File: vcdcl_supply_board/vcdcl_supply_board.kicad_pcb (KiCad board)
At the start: 2 copper layers, 30 x 50 mm, 19 parts, among them J1 Conn_01x02_Male, Q1 IRFR9024, Q2 Q_NPN_ECB, Q3 Q_NPN_BCE, SW1 SW_DIP_x01

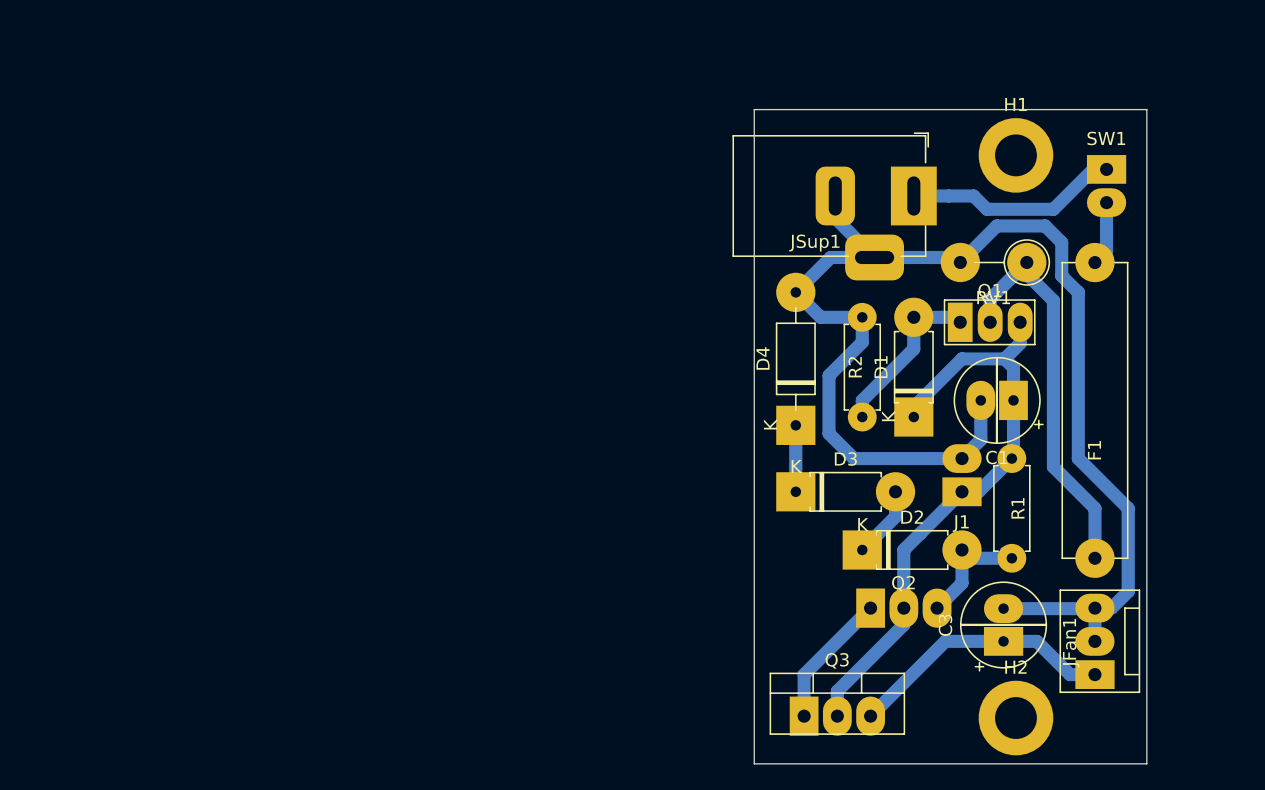
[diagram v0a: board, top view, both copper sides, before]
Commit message: Supply board fixes
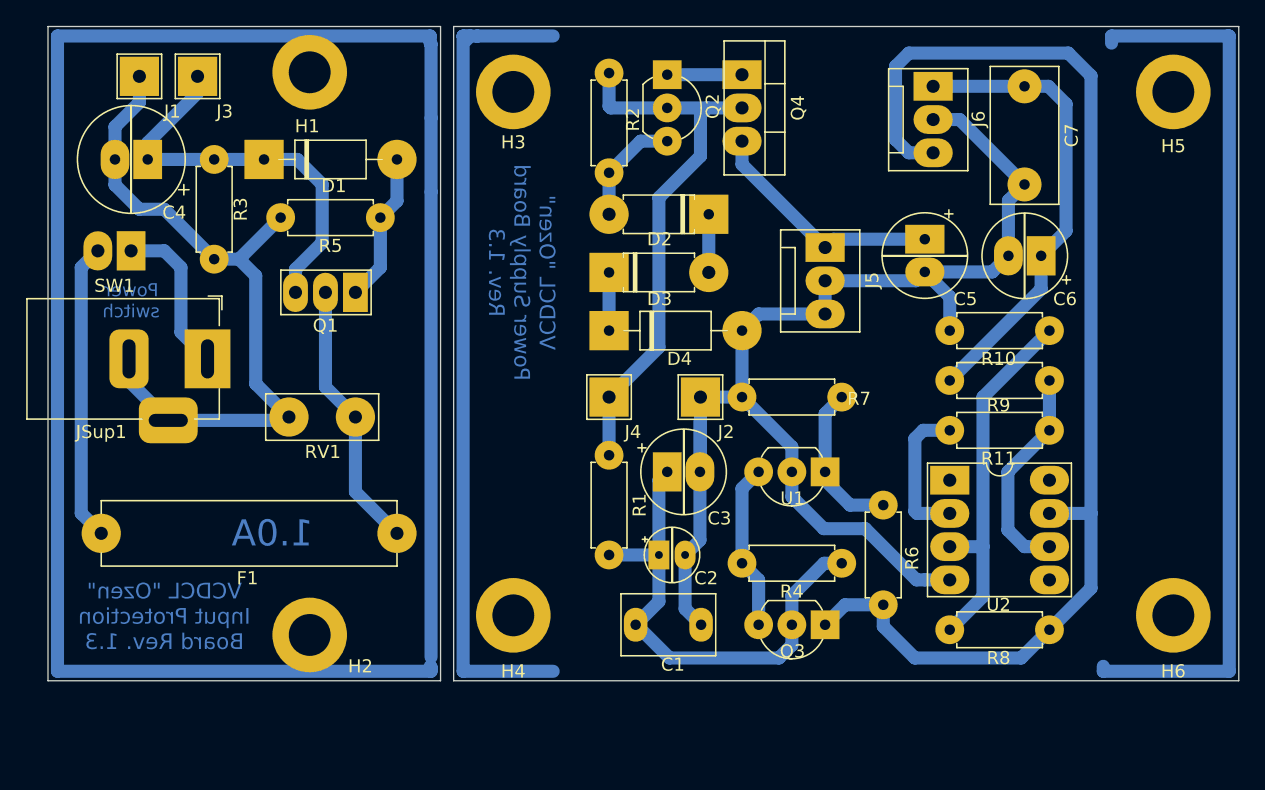
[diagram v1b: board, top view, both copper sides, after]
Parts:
- removed JFan1: Conn_01x03, _сustom:LUT_FanPinHeader_1x03_P2.54mm_Vertical
- added C2: 10u, _сustom:LUT_CP_Radial_D4.0mm_P2.00mm, F.Cu at (72.7, 64.0)
- added C4: 47u 63v, _сustom:LUT_CP_Radial_D8.0mm_P2.50mm, F.Cu at (33.6, 33.8)
- added C5: 470u 16v, _сustom:LUT_CP_Radial_D6.3mm_P2.50mm, F.Cu at (93.0, 39.9)
- added C6: 470u, _сustom:LUT_CP_Radial_D6.3mm_P2.50mm, F.Cu at (101.9, 41.2)
- added C7: 150u, _сustom:LUT_C_Rect_L10.3mm_W5.0mm_P7.50mm, F.Cu at (100.7, 28.2)
- added G***: LOGO, _сustom:Logo_Ozen_7.0x9.0, F.Cu at (62.9, 59.8)
- added G***: LOGO, _сustom:Logo_Ozen_7.0x9.0, F.Cu at (34.9, 60.5)
- added H3: MountingHole_Pad, MountingHole:MountingHole_3.2mm_M3_ISO7380_Pad, F.Cu at (61.6, 28.6)
- added H4: MountingHole_Pad, MountingHole:MountingHole_3.2mm_M3_ISO7380_Pad, F.Cu at (61.6, 68.7)
- added H5: MountingHole_Pad, MountingHole:MountingHole_3.2mm_M3_ISO7380_Pad, F.Cu at (112.0, 28.6)
- added H6: MountingHole_Pad, MountingHole:MountingHole_3.2mm_M3_ISO7380_Pad, F.Cu at (112.0, 68.7)
- added J2: Conn_01x01_Female, _сustom:LUT_PinHeader_1x01_P2.54mm_Vertical, F.Cu at (75.9, 52.0)
- added J3: Conn_01x01_Female, _сustom:LUT_PinHeader_1x01_P2.54mm_Vertical, F.Cu at (37.5, 27.5)
- added J4: Conn_01x01_Female, _сustom:LUT_PinHeader_1x01_P2.54mm_Vertical, F.Cu at (68.9, 52.0)
- added J5: Conn_01x03, _сustom:LUT_FanPinHeader_1x03_P2.54mm_Vertical, F.Cu at (85.4, 40.5)
- added J6: Conn_01x03, _сustom:LUT_FanPinHeader_1x03_P2.54mm_Vertical, F.Cu at (93.7, 28.2)
- added Q4: Q_NPN_BCE, _сustom:LUT_TO-220-3_Vertical, F.Cu at (79.1, 27.3)
- added R10: 5k 1%, _сustom:LUT_R_L6.3mm_D2.5mm_P7.62mm_Horizontal, F.Cu at (102.6, 46.9)
- added R11: 5k, _сustom:LUT_R_L6.3mm_D2.5mm_P7.62mm_Horizontal, F.Cu at (102.6, 54.5)
- added R3: 100k, _сustom:LUT_R_L6.3mm_D2.5mm_P7.62mm_Horizontal, F.Cu at (38.7, 41.4)
- added R4: 1k, _сustom:LUT_R_L6.3mm_D2.5mm_P7.62mm_Horizontal, F.Cu at (86.7, 64.7)
- added R5: 5k, _сustom:LUT_R_L6.3mm_D2.5mm_P7.62mm_Horizontal, F.Cu at (51.4, 38.3)
- added R6: 5k 1%, _сustom:LUT_R_L6.3mm_D2.5mm_P7.62mm_Horizontal, F.Cu at (89.9, 67.8)
- added R7: 1k 1%, _сustom:LUT_R_L6.3mm_D2.5mm_P7.62mm_Horizontal, F.Cu at (86.7, 52.0)
- added R8: 10k 1%, _сustom:LUT_R_L6.3mm_D2.5mm_P7.62mm_Horizontal, F.Cu at (102.6, 69.8)
- added R9: 47, _сustom:LUT_R_L6.3mm_D2.5mm_P7.62mm_Horizontal, F.Cu at (94.9, 50.7)
- added U1: TL431LP, _сustom:LUT_TO-92, F.Cu at (85.4, 57.7)
- added U2: LM741, _сustom:LUT_DIP-8, F.Cu at (94.9, 58.3)
- C1: value 100u -> 1u; footprint _сustom:LUT_CP_Radial_D6.3mm_P2.50mm -> _сustom:LUT_C_Rect_L7.0mm_W4.5mm_P5.00mm
- C3: value 470u -> 100u
- D1: footprint _сustom:LUT_D_P7.62mm_Horizontal -> _сustom:LUT_D_P10.16mm_Horizontal
- J1: value Conn_01x02_Male -> Conn_01x01_Female; footprint _сustom:LUT_PinHeader_1x02_P2.54mm_Vertical -> _сustom:LUT_PinHeader_1x01_P2.54mm_Vertical
- Q3: value Q_NPN_BCE -> Q_NPN_ECB; footprint _сustom:LUT_TO-220-3_Vertical -> _сustom:LUT_TO-92
- R1: value 1k -> R
- R2: value 10k -> 390
- moved SW1 74.8 mm to (32.4, 40.8), turned to 270 degrees
- moved J1 70.4 mm to (33.0, 27.5)
- moved JSup1 55.4 mm to (38.2, 49.0)
- moved H1 54.3 mm to (46.0, 27.1)
- moved H2 54.3 mm to (46.0, 70.2)
- moved D1 53.4 mm to (42.5, 33.8), turned to 0 degrees
- moved F1 53.4 mm to (52.7, 62.4), turned to 180 degrees
- moved RV1 52.6 mm to (49.5, 53.5)
- moved Q1 46.3 mm to (49.5, 44.0), turned to 180 degrees
- moved Q2 43.6 mm to (73.3, 27.3), turned to 270 degrees
- moved C1 33.6 mm to (70.9, 69.4), turned to 0 degrees
- moved R2 32.6 mm to (68.9, 27.2), turned to 270 degrees
- moved R1 31.7 mm to (68.9, 64.0), turned to 90 degrees
- moved C3 28.8 mm to (73.3, 57.7), turned to 0 degrees
- moved D2 28.2 mm to (76.5, 38.0), turned to 180 degrees
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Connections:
- C1 pad 1: V+ -> Net-(C1-Pad1)
- C3 pad 1: +12V -> Net-(C1-Pad1)
- D1 pad 1: V+ -> Vin
- J1 pad 1: V+ -> Earth
- Q1 pad 3: V+ -> Vin
- Q2 pad 2: V+ -> Vin
- Q3 pad 1: Net-(Q2-Pad1) -> +15V
- Q3 pad 2: V+ -> Net-(C1-Pad1)
- Q3 pad 3: +12V -> Net-(Q3-Pad3)
- R1 pad 1: V+ -> Net-(C1-Pad1)
- R1 pad 2: Net-(D2-Pad2) -> Vin
- R2 pad 1: Net-(D1-Pad2) -> Vin
- R2 pad 2: Earth -> Net-(D2-Pad2)
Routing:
- net (no net): track 0.00 -> 284.9 mm
- net +15V: track 0.00 -> 93.7 mm
- net Vin: track 0.00 -> 73.6 mm
- net Earth: track 104.4 -> 153.7 mm
- net V+: track 46.4 -> 0.00 mm
- net Net-(C1-Pad1): track 0.00 -> 38.6 mm
- net +5V: track 0.00 -> 35.5 mm
- net Net-(R10-Pad1): track 0.00 -> 28.6 mm
- net Net-(F1-Pad2): track 4.95 -> 22.7 mm
- net Net-(R11-Pad1): track 0.00 -> 16.4 mm
- net Net-(Q3-Pad3): track 0.00 -> 12.7 mm
- net Net-(R6-Pad2): track 0.00 -> 12.1 mm
- net Net-(R11-Pad2): track 0.00 -> 11.2 mm
- net Net-(F1-Pad1): track 30.5 -> 20.7 mm
- net Net-(Q2-Pad1): track 10.4 -> 5.72 mm
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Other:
- board size 30 x 50 mm -> 91 x 50 mm
- board text added: "1.0A"
- board text added: "Fan"
- board text added: "Gnd"
- board text added: "Main"
- board text added: "Power switch"
- board text added: "VCDCL "Ozen" Input Protection Board Rev. 1.3"
- board text added: "VCDCL "Ozen" Power Supply Board Rev. 1.3"
- board text added: "Vin"
